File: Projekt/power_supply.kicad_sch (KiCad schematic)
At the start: 14 parts, among them U4 AOZ1280CI, U5 LM1117-3.3

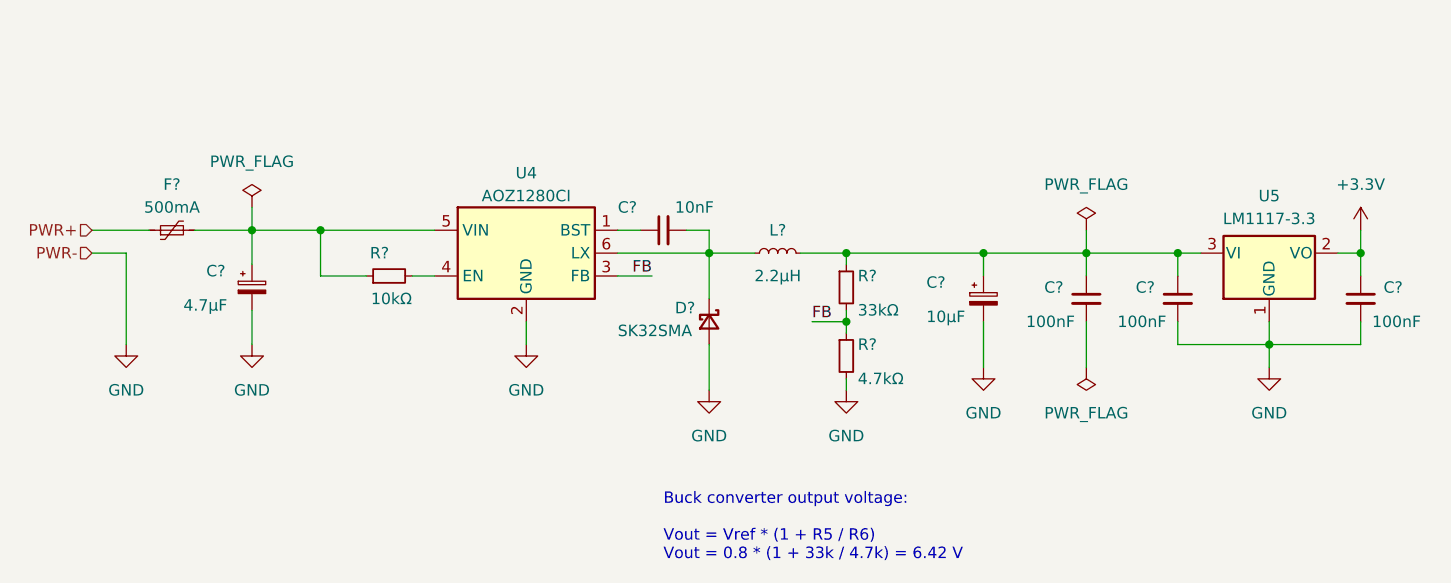
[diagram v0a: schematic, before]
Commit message: Add files via upload
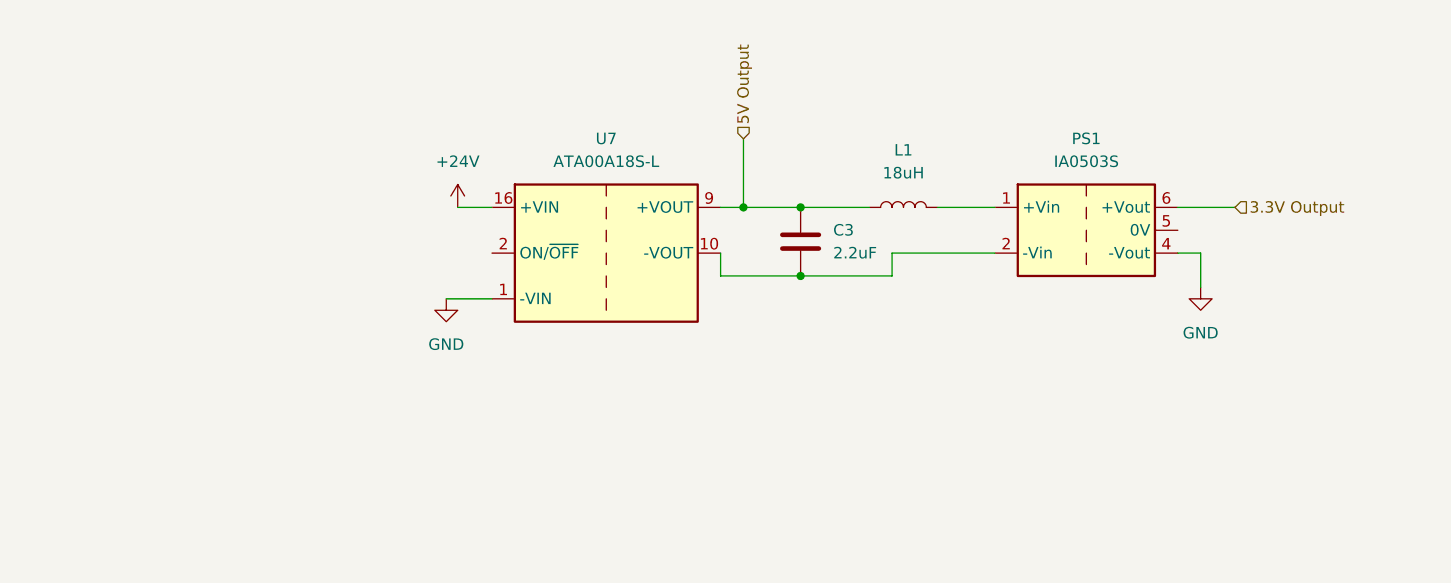
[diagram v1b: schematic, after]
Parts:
- removed C?: 10μF, Capacitor_SMD:C_Elec_4x5.4, symbol Device:C_Polarized_Small
- removed C? (x3): 100nF, Capacitor_SMD:C_0603_1608Metric, symbol Device:C_Small
- removed C?: 10nF, Capacitor_SMD:C_0603_1608Metric, symbol Device:C_Small
- removed C?: 4.7μF, Capacitor_SMD:C_Elec_4x5.4, symbol Device:C_Polarized_Small
- removed D?: SK32SMA, Diode_SMD:D_SMA, symbol Device:D_Schottky_Small
- removed F?: 500mA, Fuse:Fuse_1210_3225Metric, symbol Device:Polyfuse_Small
- removed L?: 2.2μH, Inductor_SMD:L_Bourns-SRN4018, symbol Device:L_Small
- removed R?: 10kΩ, Resistor_SMD:R_0603_1608Metric, symbol Device:R_Small
- removed R?: 4.7kΩ, Resistor_SMD:R_0603_1608Metric, symbol Device:R_Small
- removed R?: 33kΩ, Resistor_SMD:R_0603_1608Metric, symbol Device:R_Small
- removed U4: AOZ1280CI, Package_TO_SOT_SMD:SOT-23-6, symbol Regulator_Switching:AOZ1280CI
- removed U5: LM1117-3.3, Package_TO_SOT_SMD:SOT-223-3_TabPin2, symbol Regulator_Linear:LM1117-3.3
- added C3: 2.2uF, symbol Device:C
- added L1: 18uH, symbol Device:L
- added PS1: IA0503S, Converter_DCDC:Converter_DCDC_XP_POWER-IAxxxxS_THT, symbol Converter_DCDC:IA0503S
- added U7: ATA00A18S-L, Converter_DCDC:Converter_DCDC_Artesyn_ATA_SMD, symbol Converter_DCDC:ATA00A18S-L
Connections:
- net GND: now also PS1.4 (-Vout), U7.1 (-VIN)
- new net: C3.2, PS1.2 (-Vin), U7.10 (-VOUT)
- new net: L1.2, PS1.1 (+Vin)
- new net +24V: U7.16 (+VIN)
- new net 3.3V Output: PS1.6 (+Vout)
- new net 5V Output: C3.1, L1.1, U7.9 (+VOUT)
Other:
- note removed: "Buck converter output voltage: Vout = Vref * (1 + R5 / R6) Vout = 0.8 * (1 + 33k / 4.7k) = 6.42 V"
